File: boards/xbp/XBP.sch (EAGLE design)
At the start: 17 parts, among them IC1 MCP1701AT, U1 INA225

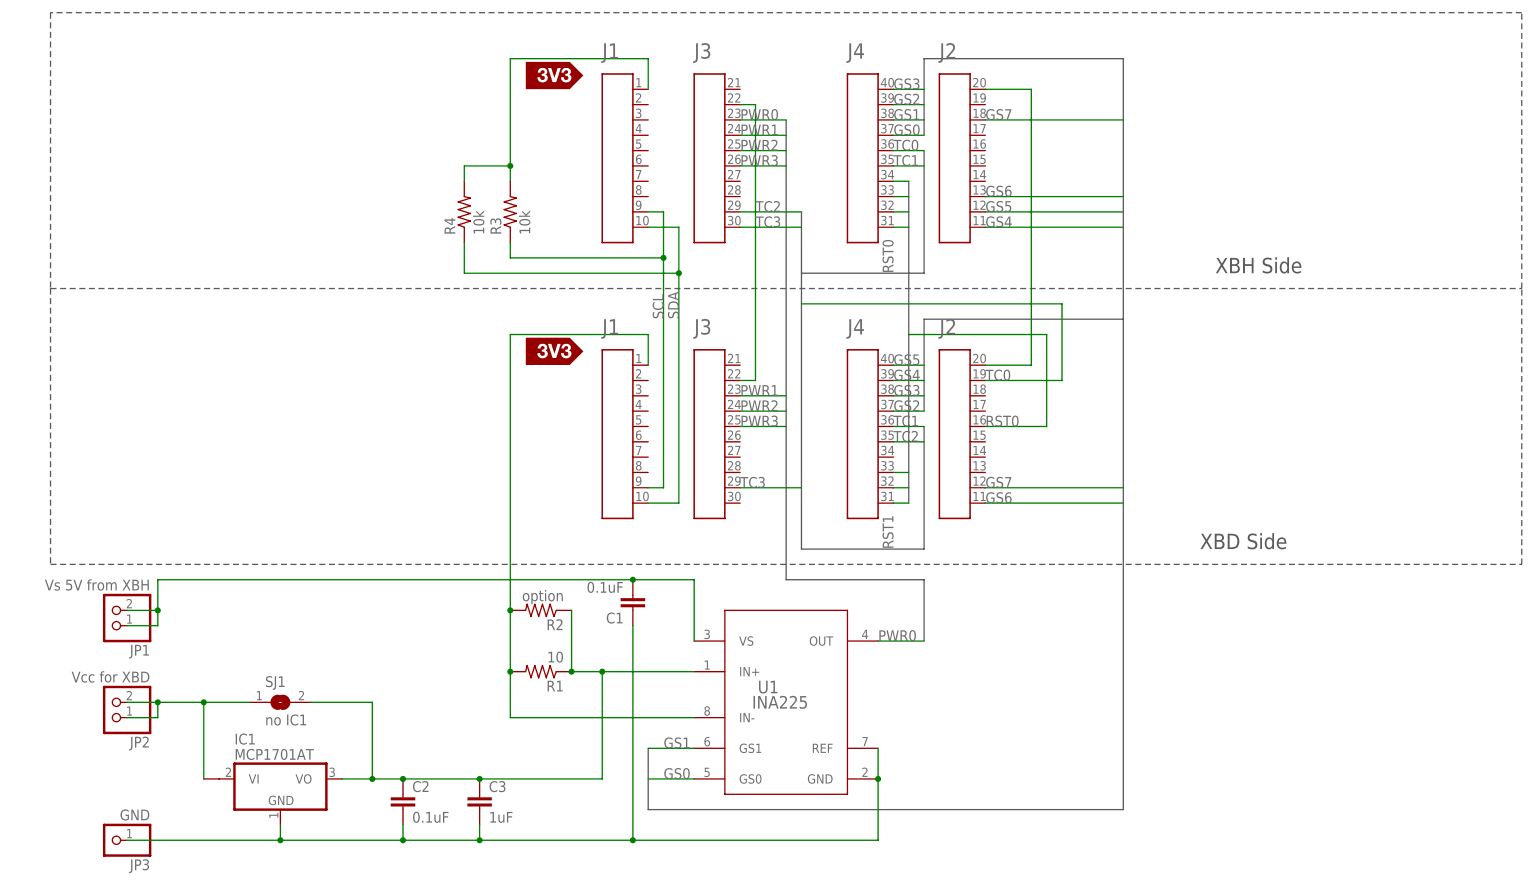
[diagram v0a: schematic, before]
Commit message: version 2.0
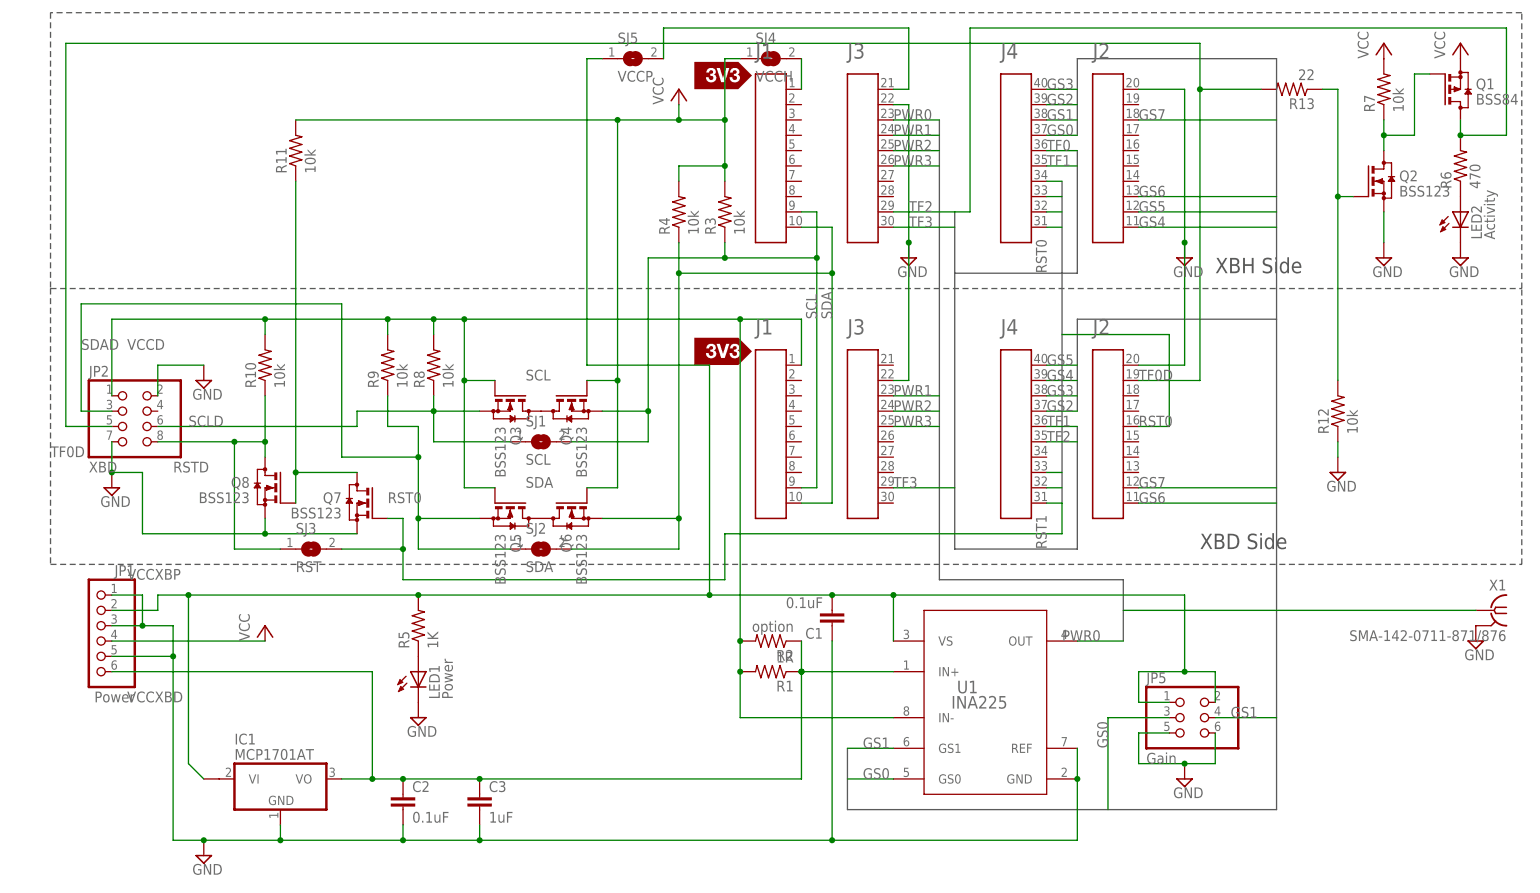
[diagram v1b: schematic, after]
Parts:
- removed JP3: GND, pinhead:PINHD-1X1
- removed U$3, U$4: SILK_3V3_TAG, Public_BP_Library:SILK_3V3_TAG
- added JP5: Gain, pinhead:PINHD-2X3
- added LED1: Power, led:LEDCHIPLED_0603
- added LED2: Activity, led:LEDCHIPLED_0603
- added Q1: BSS84, transistor-small-signal:BSS84
- added Q2, Q3, Q4, Q5, Q6, Q7, Q8: BSS123, transistor-small-signal:BSS123
- added R10, R11, R12, R7, R8, R9: 10k, resistor:R-US_R0603
- added R13: 22, resistor:R-US_R0603
- added R5: 1K, resistor:R-US_R0603
- added R6: 470, resistor:R-US_R0603
- added SJ2: SDA, jumper:SJ
- added SJ3: RST, jumper:SJ
- added SJ4: VCCH, jumper:SJ
- added SJ5: VCCP, jumper:SJ
- added U3, U4: SILK_3V3_TAG, Public_BP_Library:SILK_3V3_TAG
- added X1: SMA-142-0711-871/876, con-coax:SMA-142-0711-871/876
- A1: value (none) -> XBHCon
- A2: value (none) -> XBDCon
- JP1: value Vs 5V from XBH -> Power; device pinhead:PINHD-1X2/90 -> pinhead:PINHD-1X6/90
- JP2: value Vcc for XBD -> XBD; device pinhead:PINHD-1X2/90 -> pinhead:PINHD-2X4/90
- R1: value 10 -> 1R
- SJ1: value no IC1 -> SCL
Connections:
- net TC1 renamed TF1
- net TC2 renamed TF2
- net TC3 renamed TF3
- removed net N$6: C2.1, C3.1, IC1.VO, R1.1, R2.1, SJ1.2, U1.IN+
- removed net TC0: A1.P$36, A2.P$19
- new net N$10: Q1.G, Q2.D, R7.1
- new net N$12: Q7.D, Q8.G, R11.1
- new net N$3: LED1.A, R5.1
- new net N$7: Q3.D, Q4.D
- new net N$9: Q5.D, Q6.D
- new net RSTD: JP2.8, Q8.D, R10.1, SJ3.1
- new net SCLD: JP2.6, Q3.S, R8.1, SJ1.1
- new net SDAD: JP2.3, Q5.S, R9.1, SJ2.1
- new net TF0: A1.P$36, Q1.D, R6.2
- new net TF0D: A2.P$19, JP2.5, R13.2
- new net VCC: JP1.4, Q1.S, Q4.G, Q6.G, R11.2, R3.2, R4.2, R7.2, SJ4.1
- new net VCCD: A2.P$1, JP2.1, Q3.G, Q5.G, R1.2, R10.2, R2.2, R8.2, R9.2, U1.IN-
- new net VCCXBD: C2.1, C3.1, IC1.VO, JP1.6, R1.1, R2.1, U1.IN+
- new net VCCXBP: C1.2, IC1.VI1, JP1.2, JP5.1, JP5.2, R5.2, SJ5.1, U1.VS
- net GND: now also JP1.1, JP1.3, JP1.5, JP2.2, JP2.7, JP5.5, JP5.6, LED1.C, LED2.C, Q2.S, Q7.S, Q8.S, R12.1, X1.2; no longer JP3.1
- net GS0: now also JP5.3
- net GS1: now also JP5.4
- net N$1: now also SJ4.2; no longer R3.2, R4.2
- net N$2: now also A1.P$21, SJ5.2; no longer A2.P$1, R1.2, R2.2, U1.IN-
- net N$4: now also Q2.G, R12.2, R13.1; no longer IC1.VI1, JP2.1, JP2.2, SJ1.1
- net N$5: now also LED2.A, R6.1; no longer C1.2, JP1.1, JP1.2, U1.VS
- net PWR0: now also X1.1
- net RST0: now also Q7.G, SJ3.2
- net SCL: now also Q4.S, SJ1.2
- net SDA: now also Q6.S, SJ2.2
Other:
- note added: "rev 2.0"
- note removed: "rev 1.0"
- moved on the sheet: C1, R1, R2, R3, R4, SJ1, U1
